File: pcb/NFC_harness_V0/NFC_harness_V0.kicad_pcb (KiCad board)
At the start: 2 copper layers, 39.3 x 32 mm, 8 parts, among them IC1 ST25DV04KC-IE6S3, J3 Vin

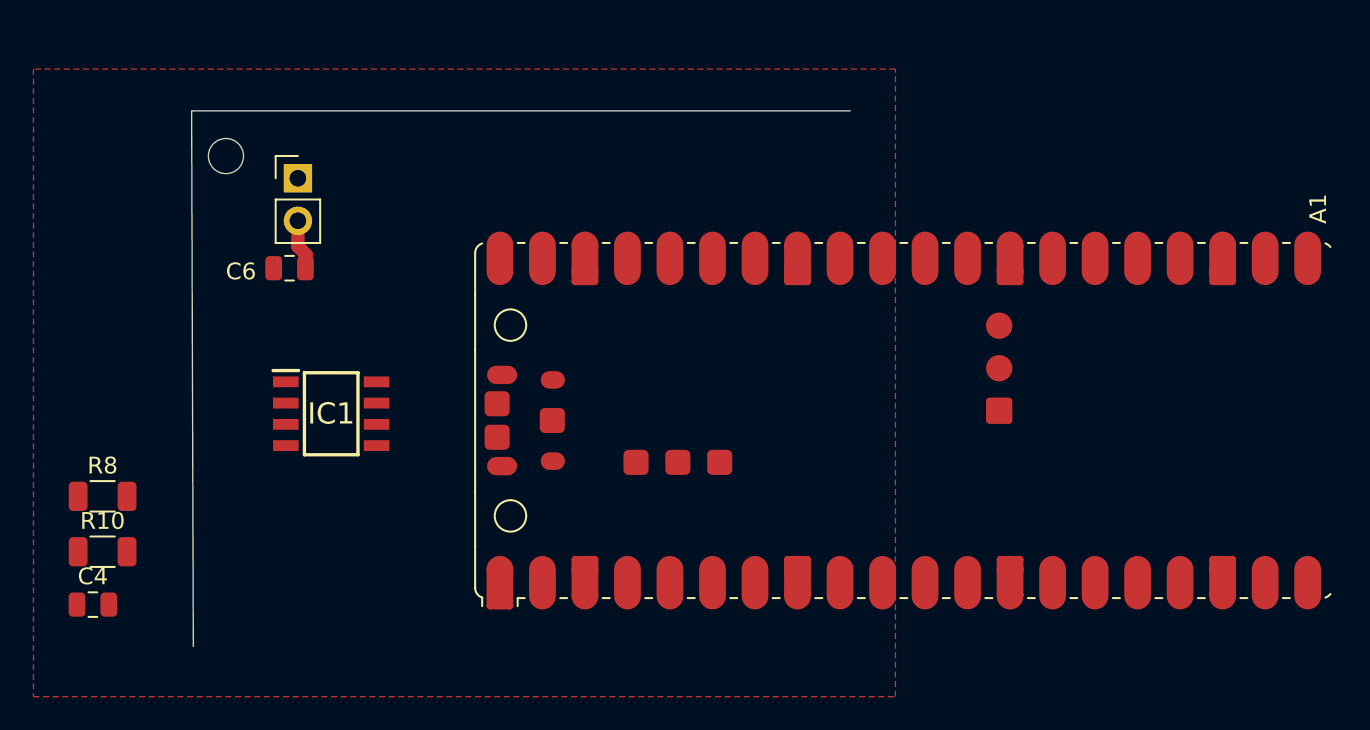
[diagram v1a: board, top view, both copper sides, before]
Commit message: pcb work
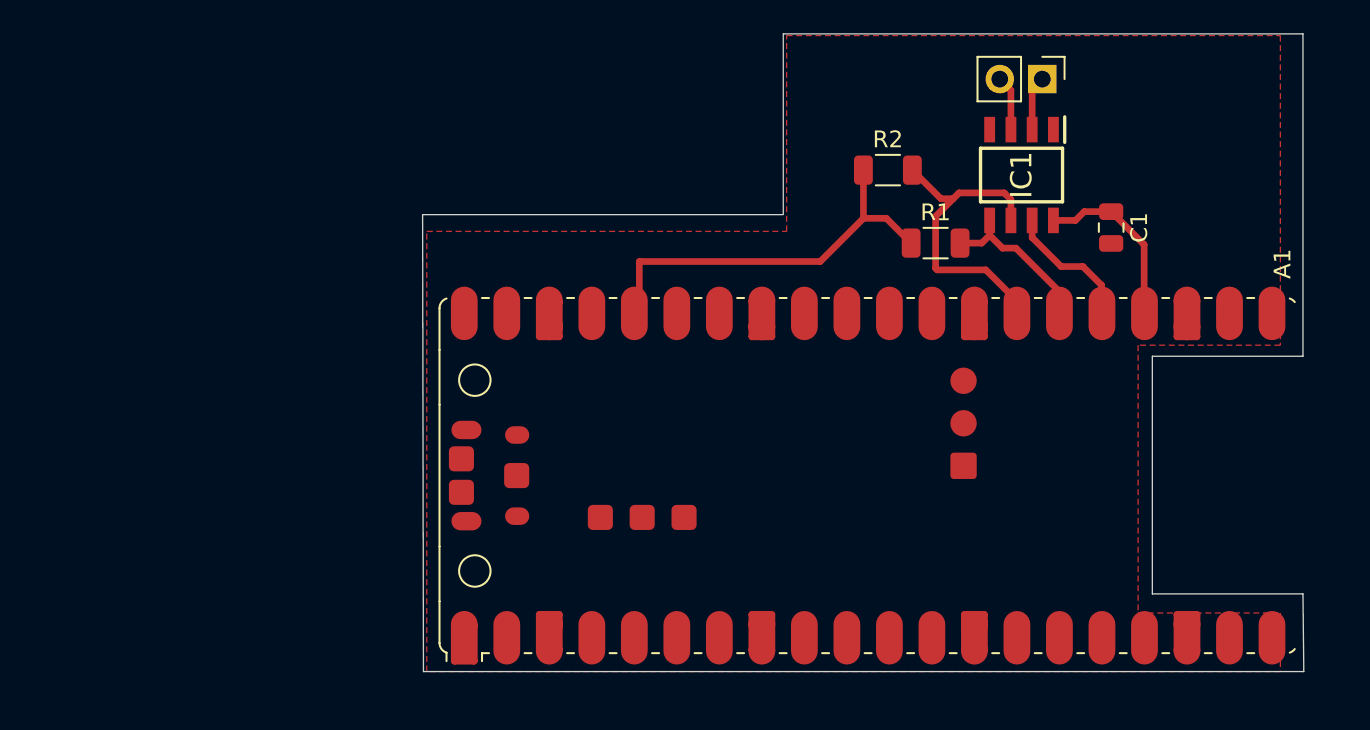
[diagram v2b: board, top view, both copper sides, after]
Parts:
- removed C4: 100n, Capacitor_SMD:C_0805_2012Metric
- removed C6: 10u, Capacitor_SMD:C_0805_2012Metric
- removed H1: MountingHole, MountingHole:MountingHole_2.1mm
- removed R10, R8: 0, Resistor_SMD:R_1206_3216Metric
- added C1: 100n, Capacitor_SMD:C_0805_2012Metric, F.Cu at (135.9, 88.0)
- added R1: 4k7, Resistor_SMD:R_1206_3216Metric, F.Cu at (125.4, 88.9)
- added R2: 4k7, Resistor_SMD:R_1206_3216Metric, F.Cu at (122.5, 84.5)
- moved J3 44.9 mm to (131.8, 79.1), turned to -90 degrees
- moved IC1 43.6 mm to (130.5, 84.8), turned to -90 degrees
- moved A1 3.92 mm to (121.4, 102.8)
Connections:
- A1 pad 13: Net-(A1-GND-Pad13) -> GND
- A1 pad 18: Net-(A1-GND-Pad13) -> GND
- A1 pad 23: Net-(A1-GND-Pad13) -> GND
- A1 pad 24: unconnected-(A1-GPIO18-Pad24) -> Net-(A1-GPIO18)
- A1 pad 25: unconnected-(A1-GPIO19-Pad25) -> Net-(A1-GPIO19)
- A1 pad 26: unconnected-(A1-GPIO20-Pad26) -> Net-(A1-GPIO20)
- A1 pad 27: unconnected-(A1-GPIO21-Pad27) -> Net-(A1-GPIO21)
- A1 pad 28: Net-(A1-GND-Pad13) -> GND
- A1 pad 3: Net-(A1-GND-Pad13) -> GND
- A1 pad 33: unconnected-(A1-AGND-Pad33) -> GND
- A1 pad 36: unconnected-(A1-3V3-Pad36) -> Net-(A1-3V3)
- A1 pad 38: Net-(A1-GND-Pad13) -> GND
- A1 pad 8: Net-(A1-GND-Pad13) -> GND
- A1 pad D2: Net-(A1-GND-Pad13) -> GND
- IC1 pad 2: unconnected-(IC1-AC0-Pad2) -> Net-(IC1-AC0)
- IC1 pad 3: unconnected-(IC1-AC1-Pad3) -> Net-(IC1-AC1)
- IC1 pad 4: unconnected-(IC1-VSS-Pad4) -> GND
- IC1 pad 5: unconnected-(IC1-SDA-Pad5) -> Net-(A1-GPIO20)
- IC1 pad 6: unconnected-(IC1-SCL-Pad6) -> Net-(A1-GPIO21)
- IC1 pad 7: unconnected-(IC1-GPO_(OPEN_DRAIN)-Pad7) -> Net-(A1-GPIO19)
- IC1 pad 8: unconnected-(IC1-VCC-Pad8) -> Net-(A1-GPIO18)
- J3 pad 1: GND -> Net-(IC1-AC0)
- J3 pad 2: Net-(J3-Pin_2) -> Net-(IC1-AC1)
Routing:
- net Net-(A1-3V3): track 0.00 -> 24.8 mm
- net Net-(A1-GPIO21): track 0.00 -> 21.6 mm
- net Net-(A1-GPIO18): track 0.00 -> 11.3 mm
- net Net-(A1-GPIO20): track 0.00 -> 10.5 mm
- net Net-(A1-GPIO19): track 0.00 -> 8.81 mm
- net Net-(IC1-AC1): track 0.00 -> 3.30 mm
- net Net-(IC1-AC0): track 0.00 -> 3.27 mm
- net Net-(J3-Pin_2): track 3.06 -> 0.00 mm
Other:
- board size 39.3 x 32 mm -> 52.7 x 38.1 mm
